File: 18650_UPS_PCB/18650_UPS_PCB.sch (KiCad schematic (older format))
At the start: 43 parts, among them J1 USB_B_Micro, J2 Conn_01x02, J3 Conn_01x02, SW1 SW_SPST, U1 STLINK-V3MINI, U10 LR9102G-xx, U11 MP2667, U2 INA237, U3 BRIGHT_TSX103, U5 STM32L151RCTx

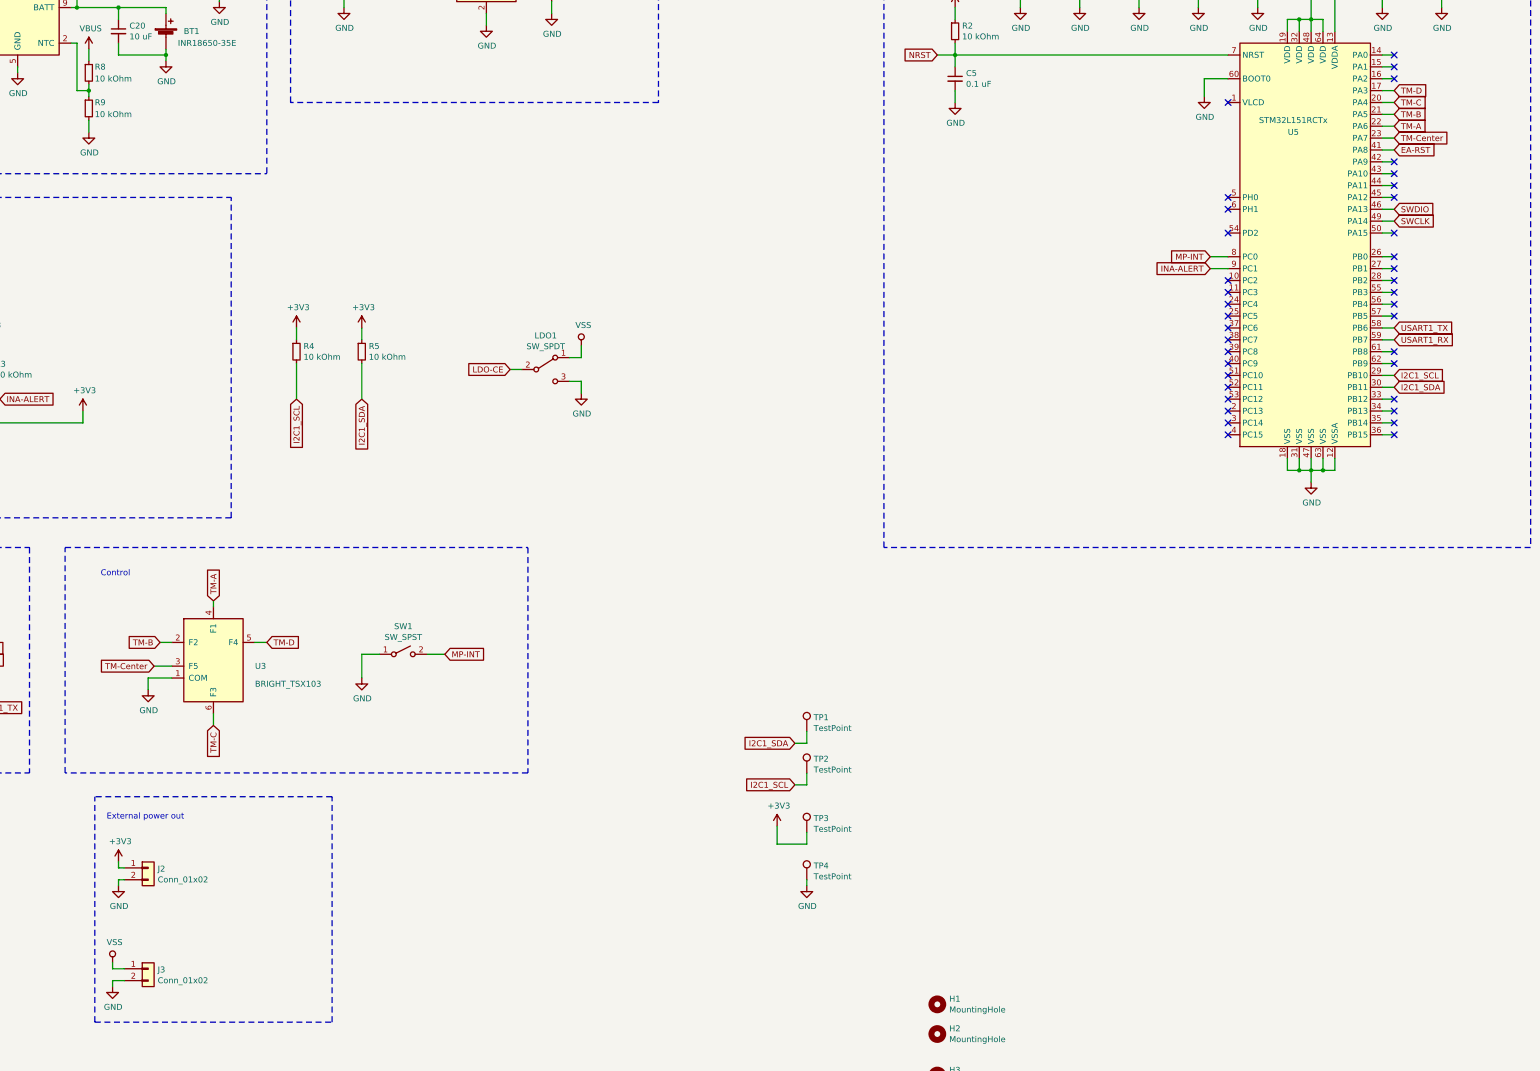
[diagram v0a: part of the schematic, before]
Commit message: Started routing V3
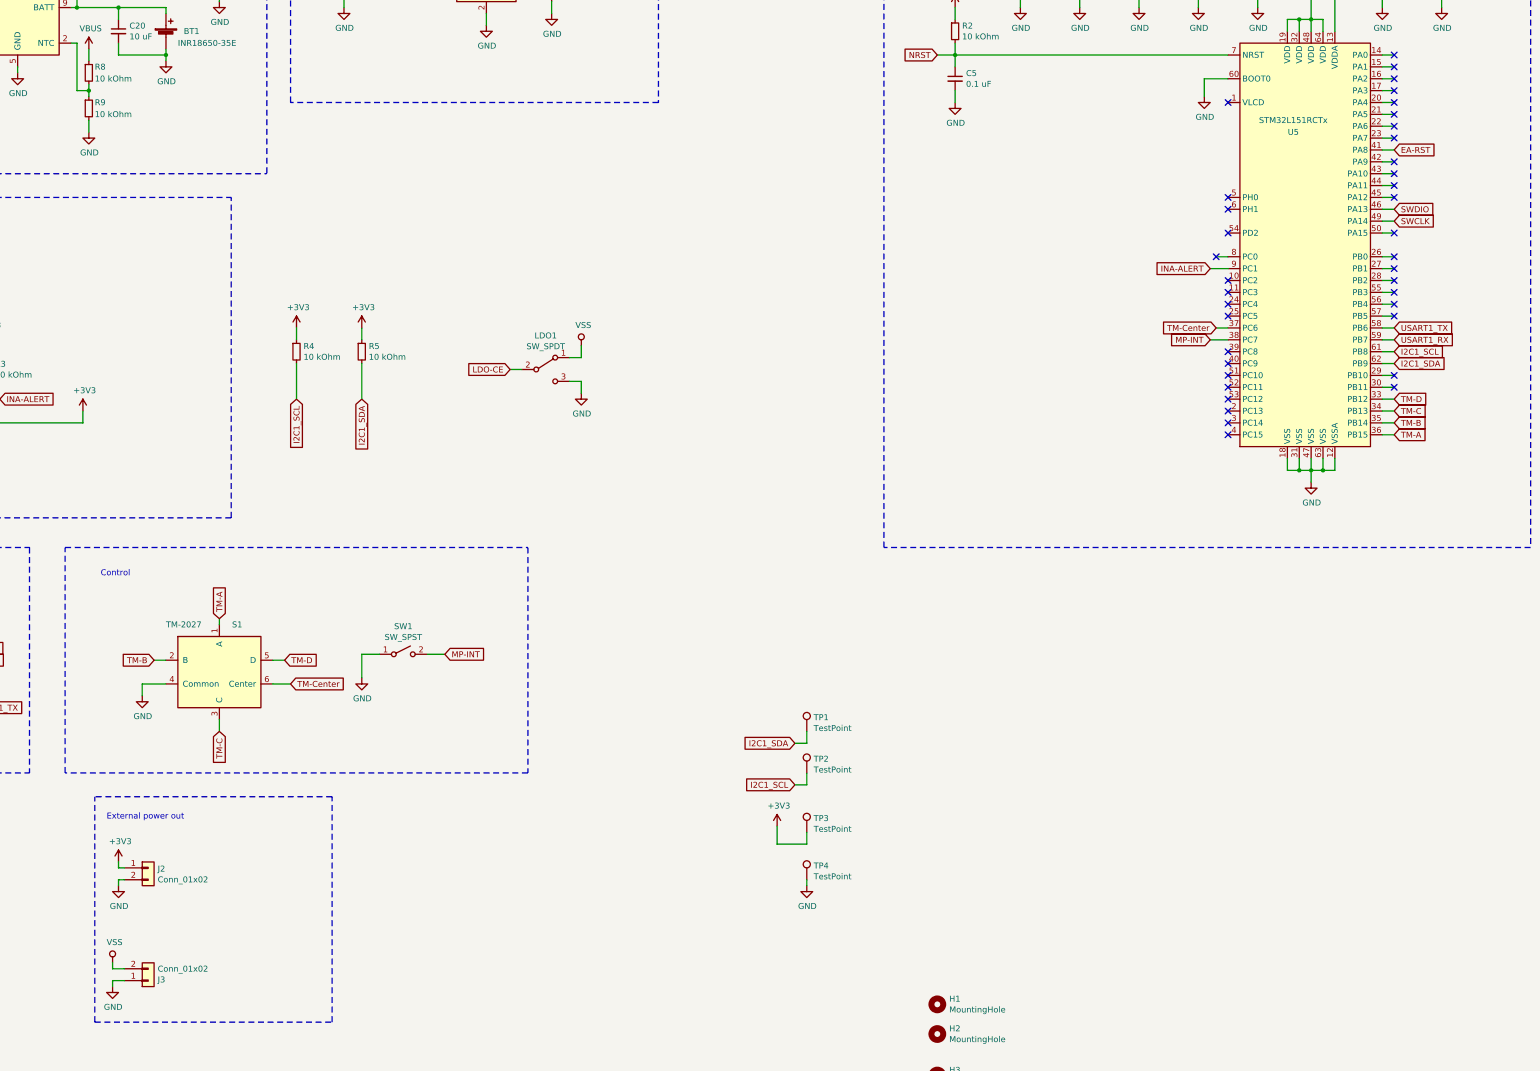
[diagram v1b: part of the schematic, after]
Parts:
- removed U3: BRIGHT_TSX103, CUSTOM_FOOTPRINTS:BRIGHT_TSX103, symbol CUSTOM_PARTS:BRIGHT_TSX103
- added S1: TM-2027, CUSTOM_FOOTPRINTS:TM-2027, symbol CUSTOM_PARTS:TM-2027
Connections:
- net GND: now also J3.1 (Pin_1), S1.4 (Common); no longer J3.2 (Pin_2)
- net I2C1_SCL: now also U5.61 (PB8); no longer U5.29 (PB10)
- net I2C1_SDA: now also U5.62 (PB9); no longer U5.30 (PB11)
- net MP-INT: now also U5.38 (PC7); no longer U5.8 (PC0)
- net TM-A: now also U5.36 (PB15), S1.1 (A); no longer U5.22 (PA6)
- net TM-B: now also U5.35 (PB14), S1.2 (B); no longer U5.21 (PA5)
- net TM-C: now also U5.34 (PB13), S1.3 (C); no longer U5.20 (PA4)
- net TM-Center: now also U5.37 (PC6), S1.6 (Center); no longer U5.23 (PA7)
- net TM-D: now also U5.33 (PB12), S1.5 (D); no longer U5.17 (PA3)
- net VSS: now also J3.2 (Pin_2); no longer J3.1 (Pin_1)
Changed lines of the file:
@@
 	1    0    0    -1
 $EndComp
-Text GLabel 13150 3750 0    50   Input ~ 0
+Text GLabel 13150 4450 0    50   Input ~ 0
 MP-INT
 Text GLabel 14700 4450 2    50   Input ~ 0
@@
 Text GLabel 14700 2850 2    50   Input ~ 0
 EA-RST
-Text GLabel 4750 6650 1    50   Input ~ 0
+Text GLabel 4800 6800 1    50   Input ~ 0
 TM-A
 Wire Wire Line
-	4750 6650 4750 6700
-Wire Wire Line
-	4400 7000 4300 7000
-Wire Wire Line
-	4750 7600 4750 7700
-Wire Wire Line
-	4400 7200 4250 7200
-Text GLabel 4300 7000 0    50   Input ~ 0
+	4800 6800 4800 6850
+Wire Wire Line
+	4350 7150 4250 7150
+Wire Wire Line
+	4800 7650 4800 7750
+Wire Wire Line
+	5250 7350 5400 7350
+Text GLabel 4250 7150 0    50   Input ~ 0
 TM-B
-Text GLabel 5200 7000 2    50   Input ~ 0
+Text GLabel 5350 7150 2    50   Input ~ 0
 TM-D
-Text GLabel 4750 7700 3    50   Input ~ 0
+Text GLabel 4800 7750 3    50   Input ~ 0
 TM-C
 $Comp
 L power:GND #PWR0123
 U 1 1 61502D4C
-P 4200 7400
-F 0 "#PWR0123" H 4200 7150 50  0001 C CNN
-F 1 "GND" H 4205 7227 50  0000 C CNN
-F 2 "" H 4200 7400 50  0001 C CNN
-F 3 "" H 4200 7400 50  0001 C CNN
-	1    4200 7400
-	1    0    0    -1
-$EndComp
-Wire Wire Line
-	4200 7300 4200 7400
-Wire Wire Line
-	4200 7300 4400 7300
-Text GLabel 14700 2650 2    50   Input ~ 0
+P 4150 7450
+F 0 "#PWR0123" H 4150 7200 50  0001 C CNN
+F 1 "GND" H 4155 7277 50  0000 C CNN
+F 2 "" H 4150 7450 50  0001 C CNN
+F 3 "" H 4150 7450 50  0001 C CNN
+	1    4150 7450
+	1    0    0    -1
+$EndComp
+Wire Wire Line
+	4150 7350 4150 7450
+Wire Wire Line
+	4150 7350 4350 7350
+Text GLabel 14700 5250 2    50   Input ~ 0
 TM-A
-Text GLabel 14700 2550 2    50   Input ~ 0
+Text GLabel 14700 5150 2    50   Input ~ 0
 TM-B
-Text GLabel 14700 2450 2    50   Input ~ 0
+Text GLabel 14700 5050 2    50   Input ~ 0
 TM-C
-Text GLabel 14700 2350 2    50   Input ~ 0
+Text GLabel 14700 4950 2    50   Input ~ 0
 TM-D
-Text GLabel 14700 2750 2    50   Input ~ 0
+Text GLabel 13200 4350 0    50   Input ~ 0
 TM-Center
 Text Notes 3800 6450 0    50   ~ 0
@@
 	14700 4450 14600 4450
 Wire Wire Line
-	14700 2750 14600 2750
-Wire Wire Line
-	14600 2650 14700 2650
-Wire Wire Line
-	14700 2550 14600 2550
-Wire Wire Line
-	14600 2450 14700 2450
-Wire Wire Line
-	14700 2350 14600 2350
-Wire Wire Line
-	13150 3750 13300 3750
+	13200 4350 13300 4350
+Wire Wire Line
+	14600 5250 14700 5250
+Wire Wire Line
+	14700 5150 14600 5150
+Wire Wire Line
+	14600 5050 14700 5050
+Wire Wire Line
+	14700 4950 14600 4950
+Wire Wire Line
+	13150 4450 13300 4450
 Wire Wire Line
 	13300 3850 13150 3850
@@
 NoConn ~ 13300 4650
 NoConn ~ 13300 4550
-NoConn ~ 13300 4450
-NoConn ~ 13300 4350
+NoConn ~ 13200 3750
+NoConn ~ 14700 2750
 NoConn ~ 13300 4250
 NoConn ~ 13300 4150
@@
 L Connector_Generic:Conn_01x02 J3
 U 1 1 610BC06E
-P 4200 9750
-F 0 "J3" H 4280 9742 50  0000 L CNN
-F 1 "Conn_01x02" H 4280 9651 50  0000 L CNN
-F 2 "CUSTOM_FOOTPRINTS:Pin_Socket_SMD_Horizontal_1x2" H 4200 9750 50  0001 C CNN
-F 3 "~" H 4200 9750 50  0001 C CNN
-	1    4200 9750
-	1    0    0    -1
+P 4200 9850
+F 0 "J3" H 4280 9842 50  0000 L CNN
+F 1 "Conn_01x02" H 4280 9751 50  0000 L CNN
+F 2 "CUSTOM_FOOTPRINTS:Pin_Socket_SMD_Horizontal_1x2" H 4200 9850 50  0001 C CNN
+F 3 "~" H 4200 9850 50  0001 C CNN
+	1    4200 9850
+	1    0    0    1
 $EndComp
 $Comp
@@
 Wire Notes Line
 	15850 700  15850 6200
-Text GLabel 14700 4850 2    50   Input ~ 0
+Text GLabel 14700 4650 2    50   Input ~ 0
 I2C1_SDA
-Text GLabel 14700 4750 2    50   Input ~ 0
+Text GLabel 14700 4550 2    50   Input ~ 0
 I2C1_SCL
 Text GLabel 5450 4950 3    50   Input ~ 0
@@
 	5450 4650 5450 4950
 Wire Wire Line
-	14700 4750 14600 4750
-Wire Wire Line
-	14600 4850 14700 4850
+	14700 4550 14600 4550
+Wire Wire Line
+	14600 4650 14700 4650
 NoConn ~ 14700 2950
 NoConn ~ 14700 3050
@@
 NoConn ~ 14700 4150
 NoConn ~ 14700 4250
-NoConn ~ 14700 4550
-NoConn ~ 14700 4650
-NoConn ~ 14700 4950
-NoConn ~ 14700 5050
-NoConn ~ 14700 5150
-NoConn ~ 14700 5250
-Wire Wire Line
-	14600 5250 14700 5250
-Wire Wire Line
-	14600 5150 14700 5150
-Wire Wire Line
-	14600 5050 14700 5050
-Wire Wire Line
-	14700 4950 14600 4950
-Wire Wire Line
-	14700 4650 14600 4650
-Wire Wire Line
-	14700 4550 14600 4550
+NoConn ~ 14700 4750
+NoConn ~ 14700 4850
+NoConn ~ 14700 2350
+NoConn ~ 14700 2450
+NoConn ~ 14700 2550
+NoConn ~ 14700 2650
+Wire Wire Line
+	14600 2650 14700 2650
+Wire Wire Line
+	14600 2550 14700 2550
+Wire Wire Line
+	14600 2450 14700 2450
+Wire Wire Line
+	14700 2350 14600 2350
+Wire Wire Line
+	14700 4850 14600 4850
+Wire Wire Line
+	14700 4750 14600 4750
 Wire Wire Line
 	14700 4250 14600 4250
@@
 Wire Wire Line
 	2250 5150 3650 5150
-$Comp
-L CUSTOM_PARTS:BRIGHT_TSX103 U3
-U 1 1 6110E704
-P 4700 6450
-F 0 "U3" H 5100 5700 50  0000 L CNN
-F 1 "BRIGHT_TSX103" H 5100 5550 50  0000 L CNN
-F 2 "CUSTOM_FOOTPRINTS:BRIGHT_TSX103" H 4650 6450 50  0001 C CNN
-F 3 "" H 4650 6450 50  0001 C CNN
-	1    4700 6450
-	1    0    0    -1
-$EndComp
-Wire Wire Line
-	5100 7000 5200 7000
+Wire Wire Line
+	5250 7150 5350 7150
 $Comp
 L Device:R_Small R6
@@
 Text GLabel 6700 7100 2    50   Input ~ 0
 MP-INT
-Text GLabel 4250 7200 0    50   Input ~ 0
+Text GLabel 5400 7350 2    50   Input ~ 0
 TM-Center
+$Comp
+L CUSTOM_PARTS:TM-2027 S1
+U 1 1 61106E72
+P 4700 6900
+F 0 "S1" H 4950 6950 50  0000 C CNN
+F 1 "TM-2027" H 4500 6950 50  0000 C CNN
+F 2 "CUSTOM_FOOTPRINTS:TM-2027" H 5550 7050 50  0001 C CNN
+F 3 "" H 5050 6900 50  0001 C CNN
+	1    4700 6900
+	1    0    0    -1
+$EndComp
+Wire Wire Line
+	14700 2750 14600 2750
+Wire Wire Line
+	13200 3750 13300 3750
 $EndSCHEMATC
